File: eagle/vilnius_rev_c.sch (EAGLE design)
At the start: 43 parts, among them IC1 PIC18F2580, IC3 MCP2551SN, IC4 LM2575S, IC5 MCP604, J1 OSTTE-12, J2 A00-108-220-450, Q1 10 MHz

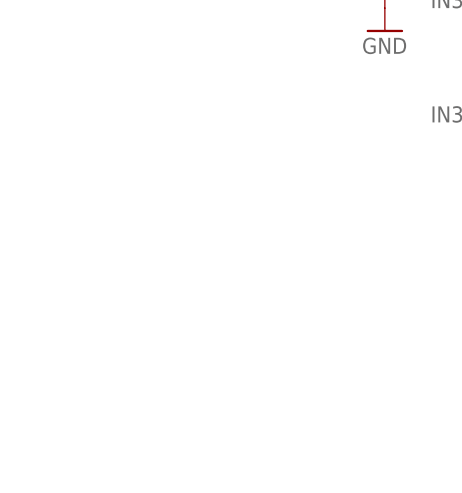
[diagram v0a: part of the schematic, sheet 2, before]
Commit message: Main functionality in place
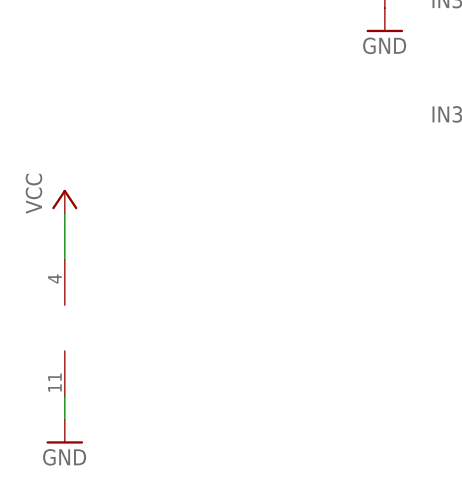
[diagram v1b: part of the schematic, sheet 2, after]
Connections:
- net GND: now also IC5P.V-
- net VCC: now also IC5P.V+
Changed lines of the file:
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@@
 <part name="R107" library="rcl" deviceset="R-EU_" device="R0805" value="10K"/>
 <part name="GND29" library="SUPPLY1" deviceset="GND" device=""/>
+<part name="P+2" library="SUPPLY1" deviceset="VCC" device=""/>
+<part name="GND18" library="SUPPLY1" deviceset="GND" device=""/>
 </parts>
 <sheets>
@@
 <instance part="R107" gate="G$1" x="116.84" y="63.5" rot="R90"/>
 <instance part="GND29" gate="1" x="116.84" y="55.88"/>
+<instance part="P+2" gate="VCC" x="60.96" y="63.5"/>
+<instance part="GND18" gate="1" x="60.96" y="35.56"/>
+<instance part="IC5" gate="P" x="60.96" y="48.26"/>
 </instances>
 <busses>
@@
 <pinref part="P+13" gate="VCC" pin="VCC"/>
 </segment>
+<segment>
+<pinref part="IC5" gate="P" pin="V+"/>
+<pinref part="P+2" gate="VCC" pin="VCC"/>
+<wire x1="60.96" y1="55.88" x2="60.96" y2="60.96" width="0.1524" layer="91"/>
+</segment>
 </net>
 <net name="GND" class="0">
@@
 <pinref part="GND29" gate="1" pin="GND"/>
 </segment>
-</net>
+<segment>
+<pinref part="IC5" gate="P" pin="V-"/>
+<pinref part="GND18" gate="1" pin="GND"/>
+<wire x1="60.96" y1="40.64" x2="60.96" y2="38.1" width="0.1524" layer="91"/>
+</segment>
+</net>
